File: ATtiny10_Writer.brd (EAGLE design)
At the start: 160 x 100 mm, 5 parts, among them CON1 AVR_ISP, J1 SOT23-6_2_SOCKET

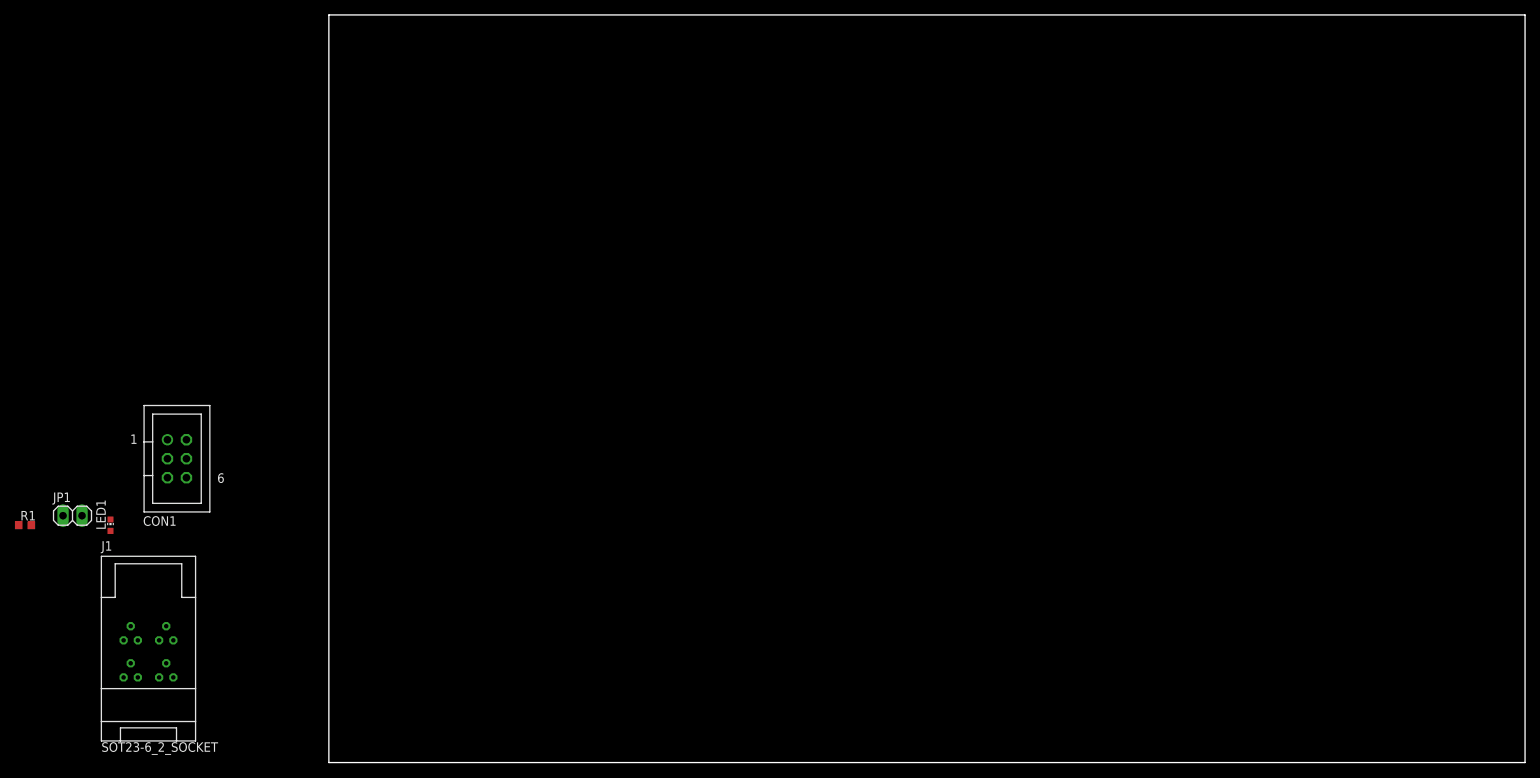
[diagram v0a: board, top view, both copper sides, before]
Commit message: complete all
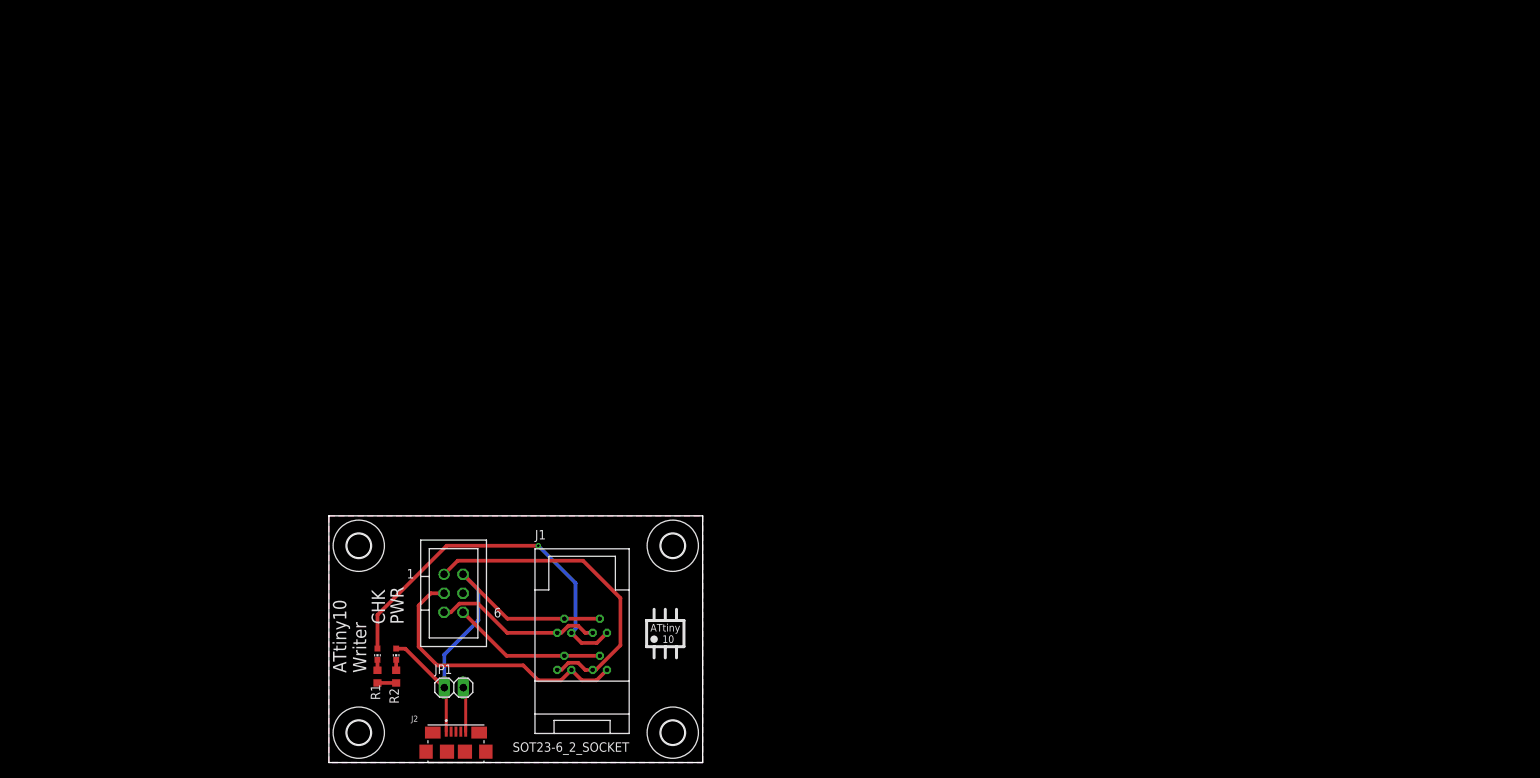
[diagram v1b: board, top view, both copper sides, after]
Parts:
- added H1, H2, H3, H4: MOUNT-HOLE3.2, holes:3,2
- added J2: ZX62-B-5PA(33), ZX62-B-5PA_33_:HRS_ZX62-B-5PA(33)
- added LED2: (no value), led:CHIP-LED0603
- added R2: (no value), rcl:R0603
- moved J1 58.0 mm to (33.9, 16.2)
- moved JP1 55.9 mm to (16.7, 10.0)
- moved R1 51.3 mm to (6.50, 11.5), turned to 90 degrees
- moved CON1 41.1 mm to (16.7, 22.6)
- moved LED1 39.7 mm to (6.50, 14.5), turned to 180 degrees
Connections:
- new net N$2: LED2.C, R2.2
- net GND: now also J2.5, J2.SH1, J2.SH2, J2.SH3, J2.SH4, J2.SH5, J2.SH6, R2.1
- net VCC: now also J2.1, LED2.A
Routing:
- net VCC: track 0.00 -> 61.4 mm
- net LED: track 0.00 -> 49.7 mm, vias 0 -> 1
- net TPIDATA: track 0.00 -> 43.3 mm
- net TPICLK: track 0.00 -> 38.4 mm
- net GND: track 0.00 -> 29.2 mm
- net RESET: track 0.00 -> 22.8 mm
- net N$2: track 0.00 -> 1.40 mm
- net N$1: track 0.00 -> 1.40 mm
- added copper zone on layer 1, net GND
- added copper zone on layer 16, net GND
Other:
- board size 160 x 100 mm -> 50 x 33 mm
- board text added: "ATtiny 10"
- board text added: "ATtiny10 Writer"
- board text added: "CHK"
- board text added: "PWR"
